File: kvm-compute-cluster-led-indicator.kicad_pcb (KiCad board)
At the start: 2 copper layers, 90 x 32.6 mm, 27 parts, among them J1 TE_1-1734248-5_FLEX, U1 PCA9685BS,118

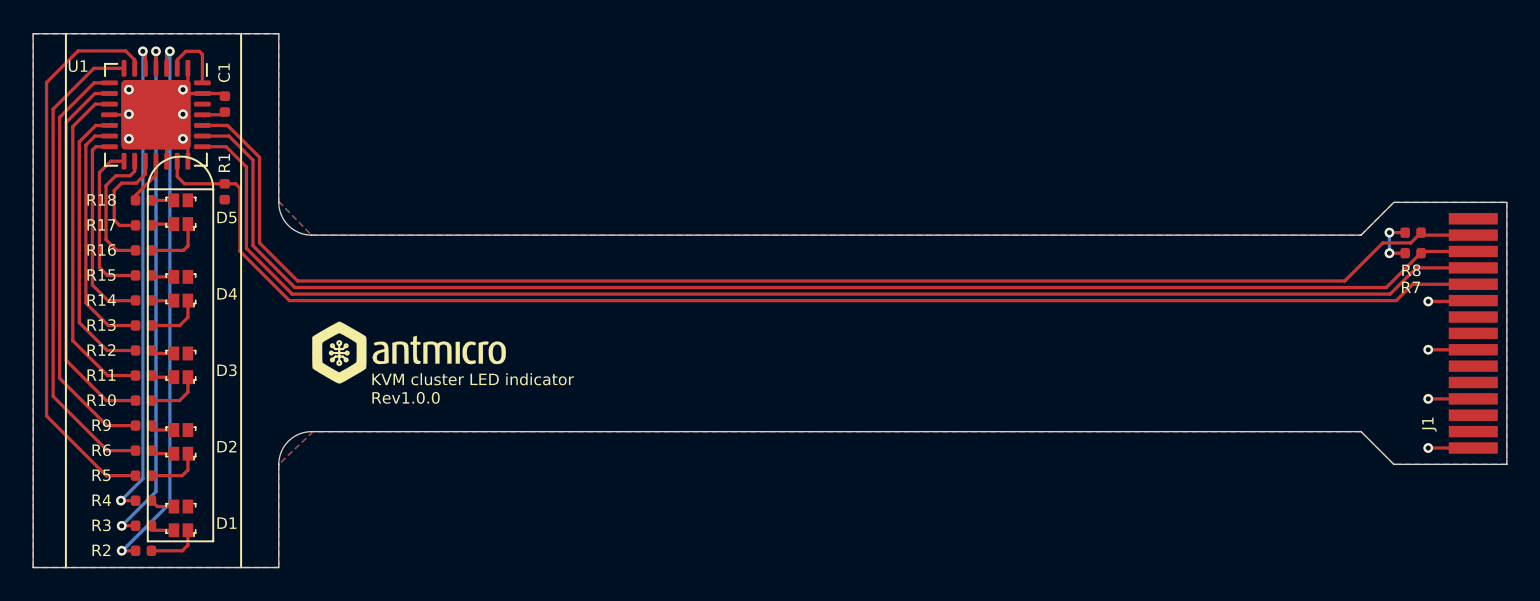
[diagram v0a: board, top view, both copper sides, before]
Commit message: Add OSHW Logo
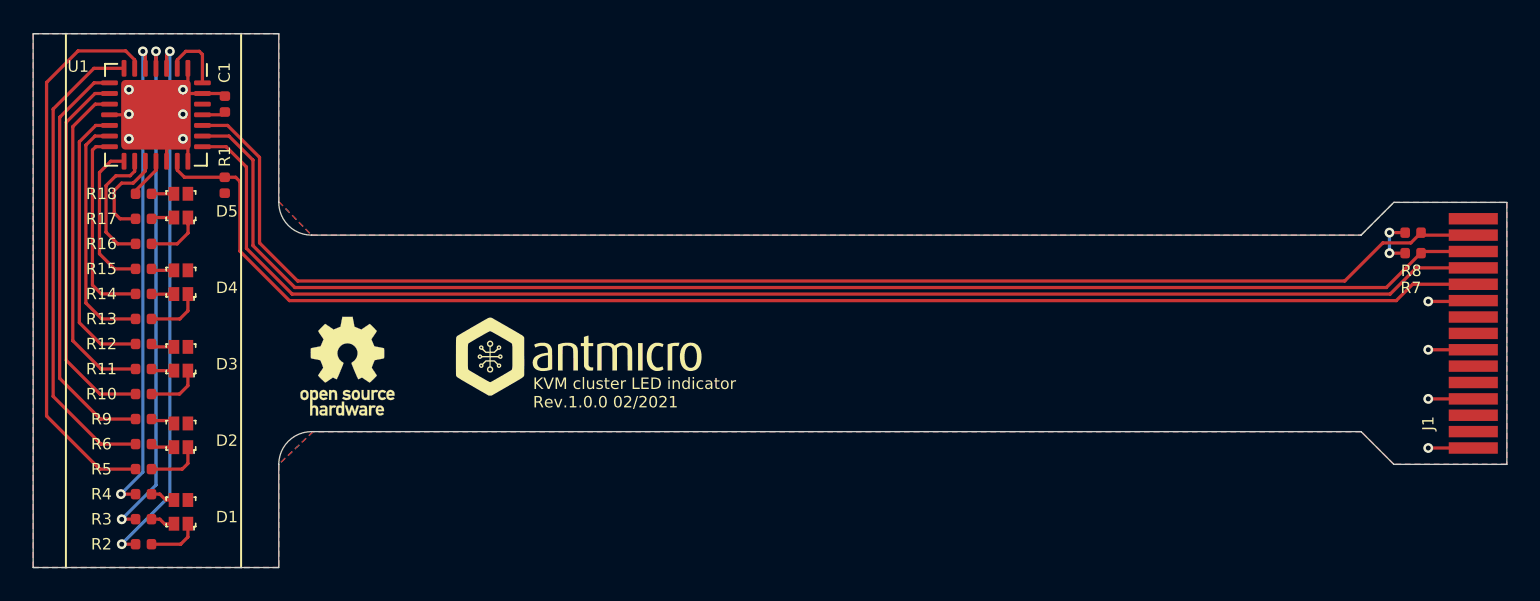
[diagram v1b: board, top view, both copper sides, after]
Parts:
- added N2: oshw_logo, antmicro-footprints:OSHW-Logo_5.7x6mm_SilkScreen, F.Cu at (117.1, 79.8)
- N1: footprint antmicro-footprints:antmicro-logo_scaled_12mm_silk -> antmicro-footprints:antmicro-logo_scaled_15mm_silk
- moved N1 10.8 mm to (131.7, 79.2)
- moved D2 0.40 mm to (106.9, 84.0)
- moved D3 0.40 mm to (106.9, 79.3)
- moved D4 0.40 mm to (106.9, 74.6)
- moved R16 0.40 mm to (104.6, 72.3)
- moved R17 0.40 mm to (104.6, 70.8)
- moved R18 0.40 mm to (104.6, 69.2)
- moved R2 0.40 mm to (104.6, 90.6)
- moved D1 0.40 mm to (106.9, 88.7)
- moved D5 0.40 mm to (106.9, 70.0)
- moved R1 0.40 mm to (109.6, 68.7)
- moved R10 0.40 mm to (104.6, 81.5)
- moved R11 0.40 mm to (104.6, 79.9)
- moved R12 0.40 mm to (104.6, 78.4)
- moved R13 0.40 mm to (104.6, 76.9)
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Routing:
- net /LED_4_B: track 9.99 -> 9.34 mm
- net Net-(D5-Pad1): track 3.68 -> 3.06 mm
- net /LED_5_G: track 6.34 -> 5.81 mm
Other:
- board text added: "KVM cluster LED indicator Rev.1.0.0 02/2021"
- board text removed: "KVM cluster LED indicator Rev1.0.0"
